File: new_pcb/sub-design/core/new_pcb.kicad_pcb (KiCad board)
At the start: 2 copper layers, 52.5 x 46.8 mm, 3 parts, among them U1 STM32F407VGTx

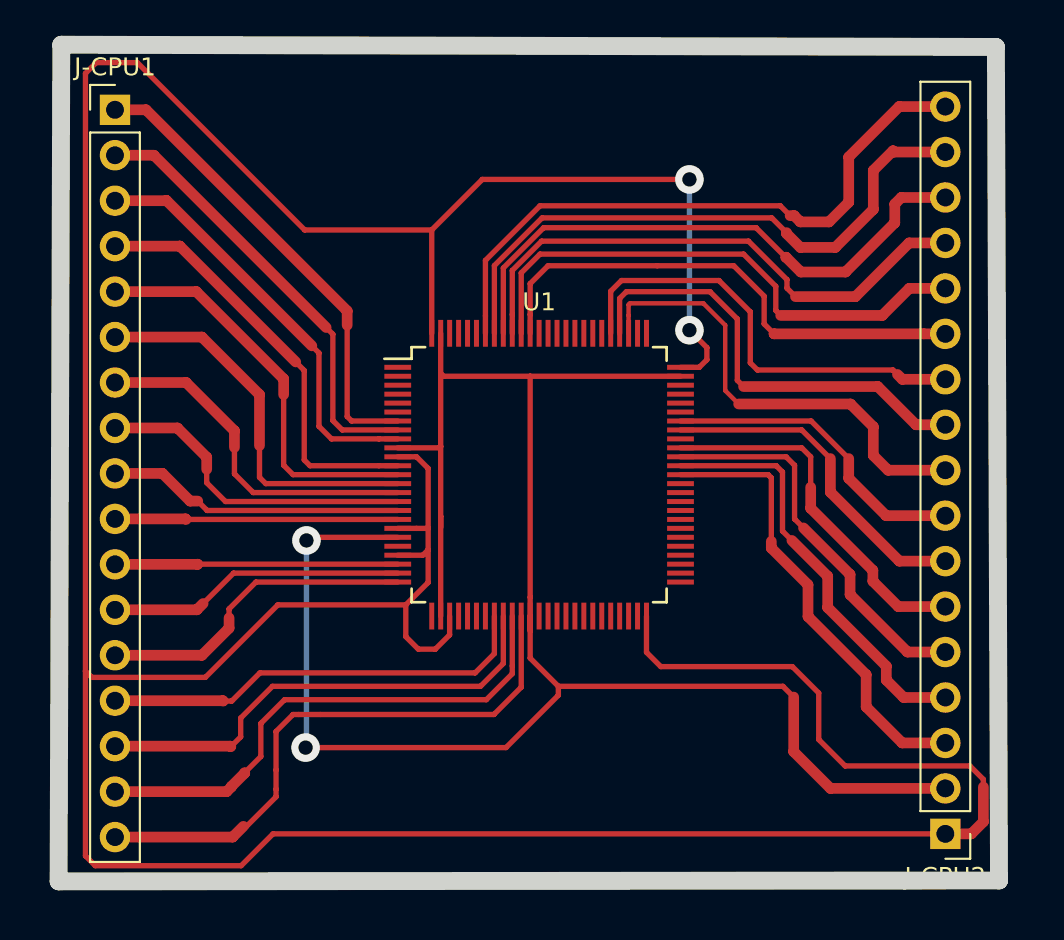
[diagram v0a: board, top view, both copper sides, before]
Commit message: progress
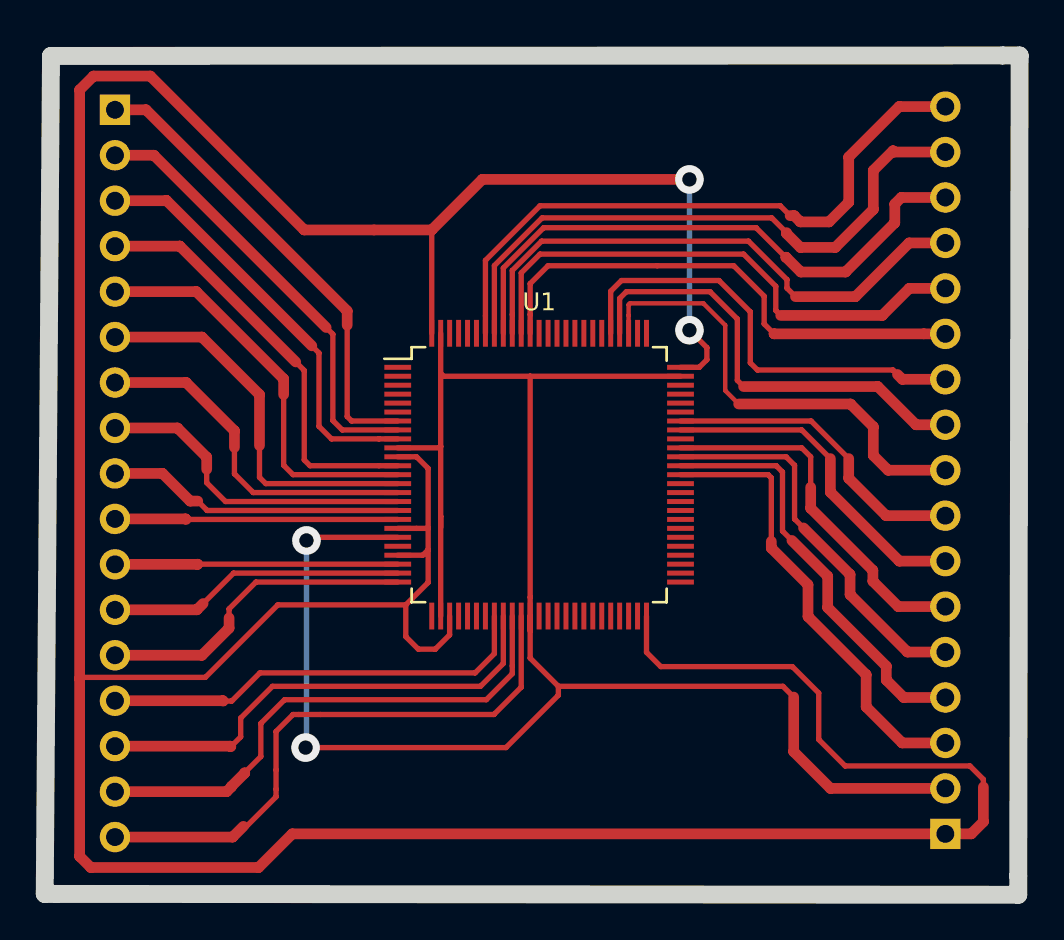
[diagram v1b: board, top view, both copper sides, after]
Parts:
- J-CPU1, J-CPU2: moved to B.Cu
- turned J-CPU1 to 180 degrees
- turned J-CPU2 to 0 degrees
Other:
- board size 52.5 x 46.8 mm -> 54.5 x 46.9 mm
